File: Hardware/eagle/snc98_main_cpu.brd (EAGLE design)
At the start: 168.2 x 30 mm, 89 parts, among them IC1 MCP170333MB, M1 IRLML2244, M12 IRLML2244, M2 IRLML2244, M3 IRLML2244, T1 BCR135, T2 BCR135, T3 BCR185, U1 74HC4051_MUX, U2 DS18B20, U3 ATMEGA1284P-PU, U4 TLV70033 / TC1185, Y2 12MHz

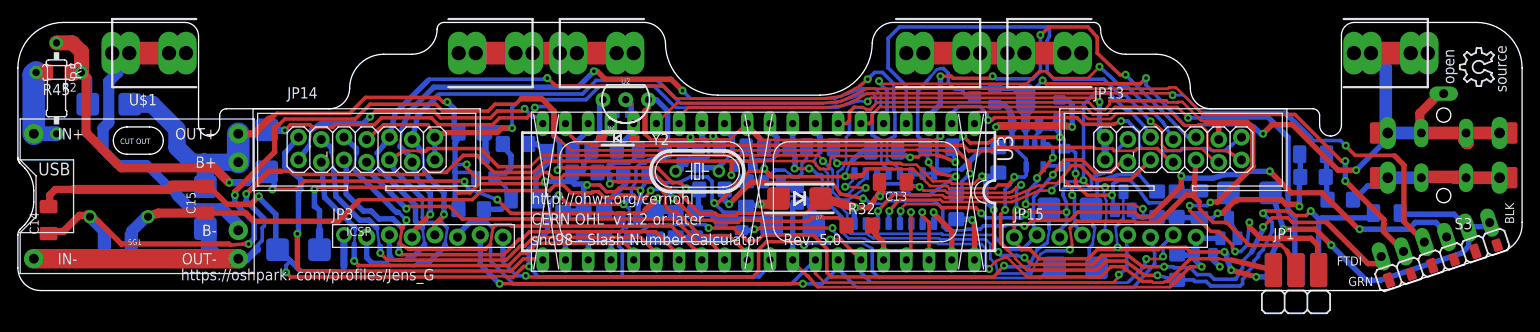
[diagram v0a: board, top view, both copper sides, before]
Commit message: sinh()_cosh()_tanh() added
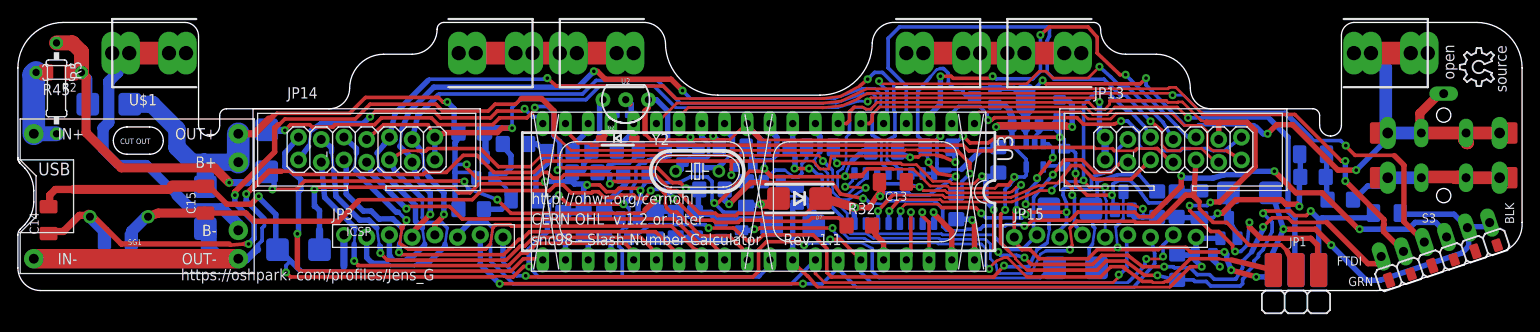
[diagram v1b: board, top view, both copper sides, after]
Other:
- board text added: "snc98 - Slash Number Calculator Rev. 1.1"
- board text removed: "snc98 - Slash Number Calculator Rev. 5.0"
